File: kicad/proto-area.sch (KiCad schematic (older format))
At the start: 4 parts, among them SW1 Reset, U4 proto-area

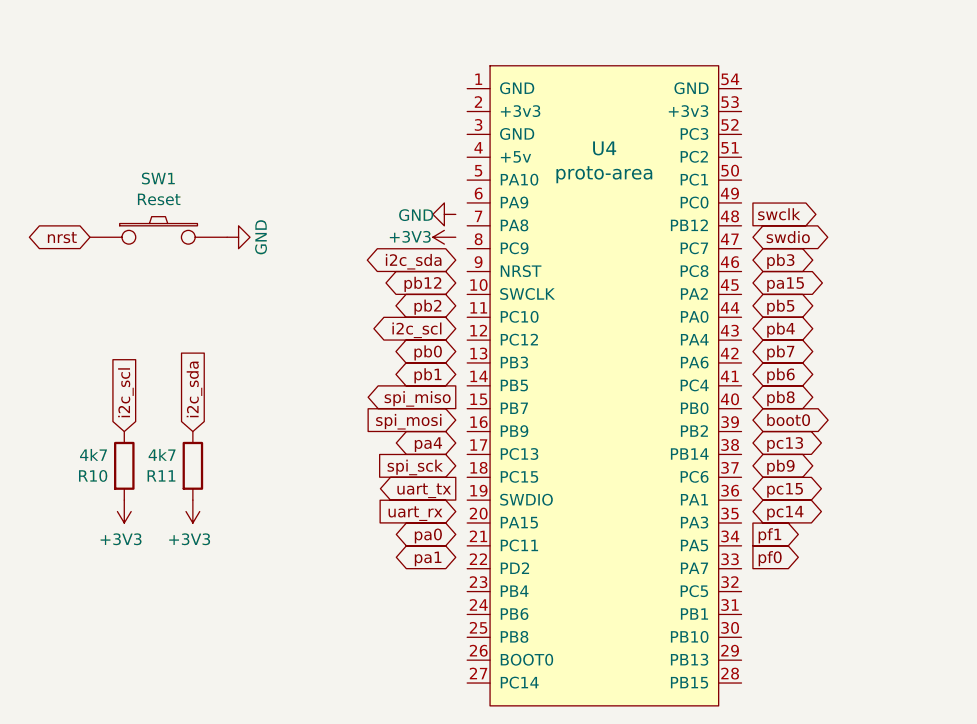
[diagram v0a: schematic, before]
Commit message: Krieger_v2.00
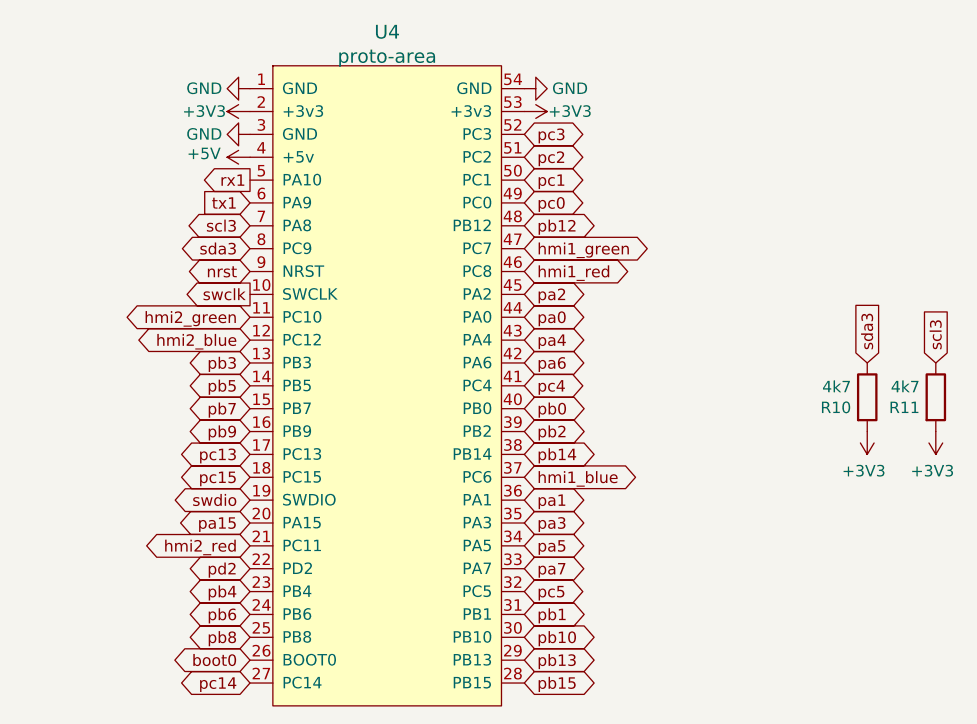
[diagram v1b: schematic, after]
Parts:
- removed SW1: Reset, krieger:TACT-SWITCH, symbol krieger:TACT-SWITCH
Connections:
- net i2c_scl is gone; now on net sda3: R10.1
- net i2c_sda is gone; now on net scl3: R11.1
- net +3V3: now also U4.2 (+3v3), U4.53 (+3v3)
- net GND: now also U4.1 (GND), U4.3 (GND), U4.54 (GND)
- net boot0: now also U4.26 (BOOT0)
- net nrst: now also U4.9 (NRST)
- net pa0: now also U4.44 (PA0)
- net pa1: now also U4.36 (PA1)
- net pa15: now also U4.20 (PA15)
- net pa4: now also U4.43 (PA4)
- net pb0: now also U4.40 (PB0)
- net pb1: now also U4.31 (PB1)
- net pb12: now also U4.48 (PB12)
- net pb2: now also U4.39 (PB2)
- net pb3: now also U4.13 (PB3)
- net pb4: now also U4.23 (PB4)
- net pb5: now also U4.14 (PB5)
- net pb6: now also U4.24 (PB6)
- net pb7: now also U4.15 (PB7)
- net pb8: now also U4.25 (PB8)
- net pb9: now also U4.16 (PB9)
- net pc13: now also U4.17 (PC13)
- net pc14: now also U4.27 (PC14)
- net pc15: now also U4.18 (PC15)
- net swclk: now also U4.10 (SWCLK)
- net swdio: now also U4.19 (SWDIO)
- net hmi2_green: now reaches U4.11 (PC10)
- net hmi2_blue: now reaches U4.12 (PC12)
- net hmi2_red: now reaches U4.21 (PC11)
- net pd2: now reaches U4.22 (PD2)
- net pb15: now reaches U4.28 (PB15)
- net pb13: now reaches U4.29 (PB13)
- net pb10: now reaches U4.30 (PB10)
- net pc5: now reaches U4.32 (PC5)
- net pa7: now reaches U4.33 (PA7)
- net pa5: now reaches U4.34 (PA5)
- net pa3: now reaches U4.35 (PA3)
- net hmi1_blue: now reaches U4.37 (PC6)
- net pb14: now reaches U4.38 (PB14)
- net +5V: now reaches U4.4 (+5v)
- net pc4: now reaches U4.41 (PC4)
- net pa6: now reaches U4.42 (PA6)
- net pa2: now reaches U4.45 (PA2)
- net hmi1_red: now reaches U4.46 (PC8)
- net hmi1_green: now reaches U4.47 (PC7)
- net pc0: now reaches U4.49 (PC0)
- net rx1: now reaches U4.5 (PA10)
- net pc1: now reaches U4.50 (PC1)
- net pc2: now reaches U4.51 (PC2)
- net pc3: now reaches U4.52 (PC3)
- net tx1: now reaches U4.6 (PA9)
- net scl3: now reaches U4.7 (PA8)
- net sda3: now reaches U4.8 (PC9)
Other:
- moved on the sheet: R10, R11

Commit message: Krieger v2.00
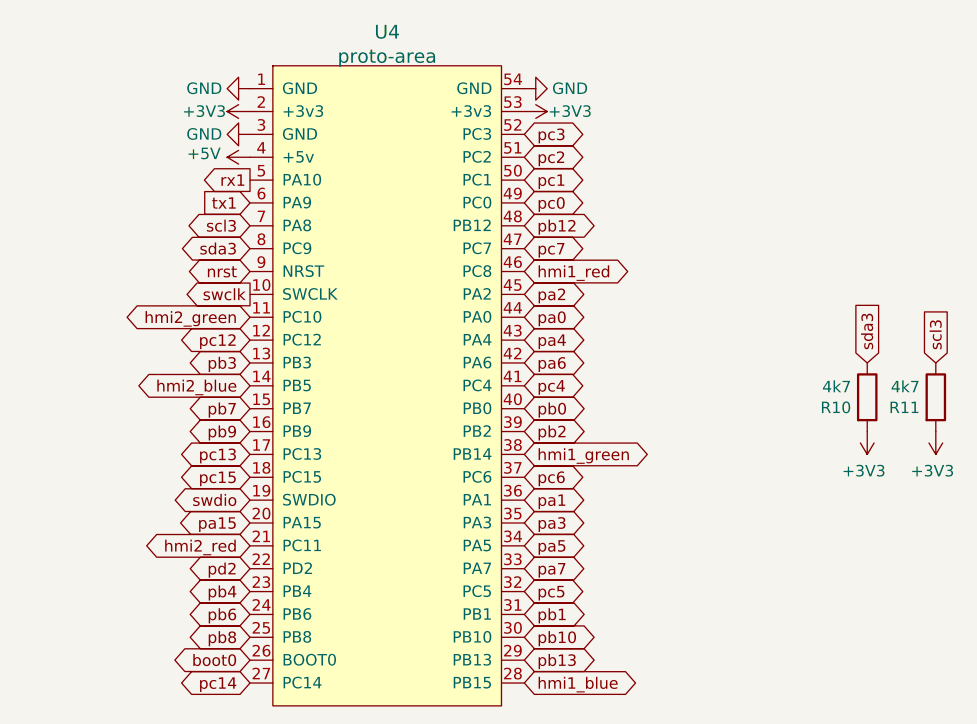
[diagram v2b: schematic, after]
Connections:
- net pb14 is gone; now on net hmi1_green: U4.38 (PB14)
- net pb15 is gone; now on net hmi1_blue: U4.28 (PB15)
- net pb5 is gone; now on net hmi2_blue: U4.14 (PB5)
- net hmi1_blue: no longer U4.37 (PC6)
- net hmi1_green: no longer U4.47 (PC7)
- net hmi2_blue: no longer U4.12 (PC12)
- new net pc12: U4.12 (PC12)
- new net pc6: U4.37 (PC6)
- new net pc7: U4.47 (PC7)
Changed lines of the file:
@@
 Sheet 3 3
 Title "Krieger"
-Date "2021-05-24"
+Date "2021-06-05"
 Rev "v2.0"
 Comp "www.2-0.dk"
@@
 Text GLabel 6200 5050 2    50   BiDi ~ 0
 pb10
-Text GLabel 5000 3950 0    50   BiDi ~ 0
-pb5
+Text GLabel 5000 3750 0    50   BiDi ~ 0
+pc12
 Text GLabel 5000 3850 0    50   BiDi ~ 0
 pb3
@@
 Text GLabel 6200 5150 2    50   BiDi ~ 0
 pb13
-Text GLabel 6200 4250 2    50   BiDi ~ 0
-pb14
-Text GLabel 6200 5250 2    50   BiDi ~ 0
-pb15
-Text GLabel 6200 3450 2    50   BiDi ~ 0
-hmi1_red
+Text GLabel 6200 3350 2    50   BiDi ~ 0
+pc7
+Text GLabel 6200 4350 2    50   BiDi ~ 0
+pc6
 Text GLabel 6200 3150 2    50   BiDi ~ 0
 pc0
@@
 	0    -1   -1   0
 $EndComp
-Text GLabel 6200 3350 2    50   BiDi ~ 0
-hmi1_green
 $Comp
 L krieger:proto-area U4
 U 1 1 6097F86E
 P 5600 3950
+AR Path="/6097F86E" Ref="U4"  Part="1"
+AR Path="/5B673B54/6097F86E" Ref="U4"  Part="1"
 F 0 "U4" H 5600 5497 60  0000 C CNN
 F 1 "proto-area" H 5600 5391 60  0000 C CNN
@@
 	1    0    0    -1
 $EndComp
-Text GLabel 6200 4350 2    50   BiDi ~ 0
+Text GLabel 6200 5250 2    50   BiDi ~ 0
 hmi1_blue
 Text GLabel 5000 3450 0    50   BiDi ~ 0
 nrst
-Text GLabel 5000 3750 0    50   BiDi ~ 0
+Text GLabel 5000 3950 0    50   BiDi ~ 0
 hmi2_blue
+Text GLabel 6200 4250 2    50   BiDi ~ 0
+hmi1_green
+Text GLabel 6200 3450 2    50   BiDi ~ 0
+hmi1_red
 $EndSCHEMATC
